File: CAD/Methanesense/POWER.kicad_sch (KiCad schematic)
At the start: 22 parts, among them J1 USB_C_Receptacle_USB2.0_14P, SW3 KMR223GLFG, U1 AP63205WU, U3 nPM1300-QEXX, U4 AP131-20, U7 FT230XQ

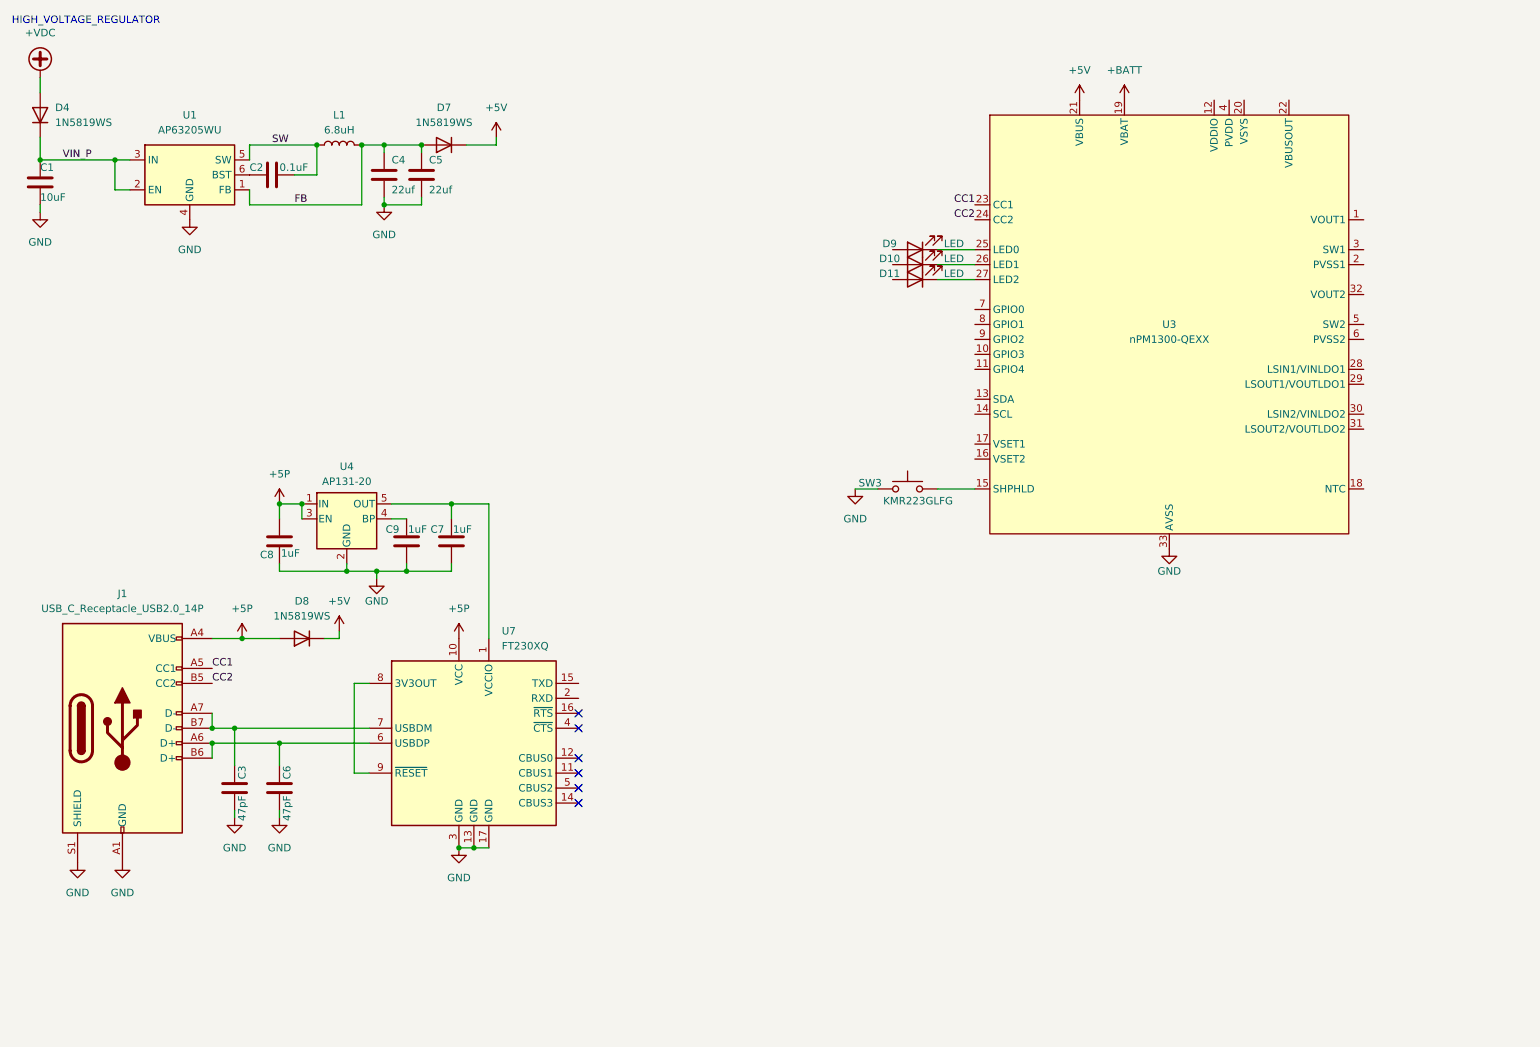
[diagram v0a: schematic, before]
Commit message: WIP
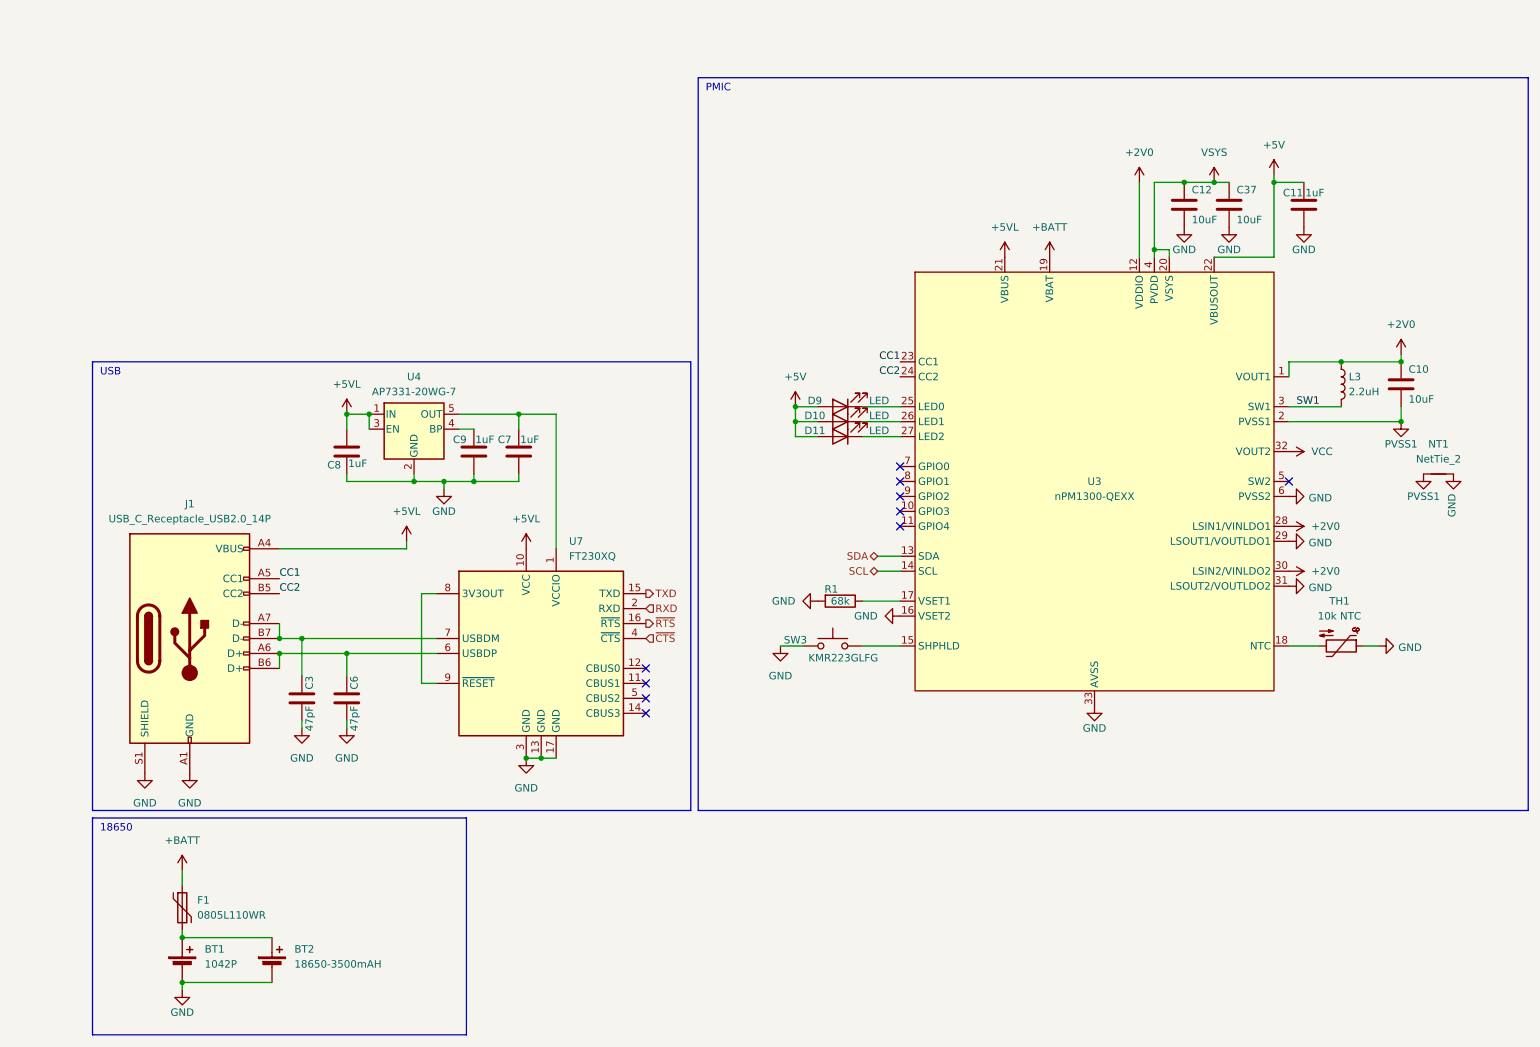
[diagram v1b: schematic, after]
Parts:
- removed C1: 10uF, Capacitor_SMD:C_0805_2012Metric, symbol Library:C
- removed C2: 0.1uF, Capacitor_SMD:C_0402_1005Metric, symbol Library:C
- removed C4, C5: 22uf, Capacitor_SMD:C_0402_1005Metric, symbol Library:C
- removed D4, D7, D8: 1N5819WS, Diode_SMD:D_SOD-323, symbol Library:1N4148WS
- removed L1: 6.8uH, Inductor_SMD:L_1008_2520Metric, symbol Device:L
- removed U1: AP63205WU, Package_TO_SOT_SMD:TSOT-23-6, symbol Regulator_Switching:AP63201WU
- added BT1: 1042P, Battery:BatteryHolder_MPD_BH-18650-PC2, symbol Device:Battery_Cell
- added BT2: 18650-3500mAH, symbol Device:Battery_Cell
- added C10, C12, C37: 10uF, Capacitor_SMD:C_0805_2012Metric, symbol Library:C
- added C11: 1uF, Capacitor_SMD:C_0603_1608Metric, symbol Library:C
- added F1: 0805L110WR, Resistor_SMD:R_1206_3216Metric, symbol Device:Polyfuse
- added L3: 2.2uH, Inductor_SMD:L_1008_2520Metric, symbol Device:L
- added NT1: NetTie_2, esprelay:Viatie, symbol Device:NetTie_2
- added R1: 68k, Resistor_SMD:R_0603_1608Metric, symbol Library:R
- added TH1: 10k NTC, Resistor_SMD:R_0603_1608Metric, symbol Device:Thermistor_NTC
- C3, C6, C7, C8, C9: footprint Capacitor_SMD:C_0402_1005Metric -> Capacitor_SMD:C_0603_1608Metric
- D10, D11, D9: footprint (none) -> LED_SMD:LED_0603_1608Metric
- J1: footprint (none) -> Methanesense:USB_C_Receptacle_HCTL_HC-TYPE-C-16P-01A
- U4: value AP131-20 -> AP7331-20WG-7
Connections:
- net +5V: now also D10.2 (A), D11.2 (A), D9.2 (A), U3.22 (VBUSOUT), C11.1; no longer U3.21 (VBUS)
- net +BATT: now also F1.1
- net GND: now also U3.16 (VSET2), U3.29 (LSOUT1/VOUTLDO1), U3.31 (LSOUT2/VOUTLDO2), U3.6 (PVSS2), BT1.2 (-), BT2.2 (-), C11.2, C12.2, C37.2, NT1.2, R1.2, TH1.1
- net TXD: now reaches U7.15 (TXD)
- net ~{RTS}: now reaches U7.16 (~{RTS})
- net RXD: now reaches U7.2 (RXD)
- net ~{CTS}: now reaches U7.4 (~{CTS})
- net +2V0: now reaches U3.1 (VOUT1)
- net +2V0: now also U3.12 (VDDIO), U3.28 (LSIN1/VINLDO1), U3.30 (LSIN2/VINLDO2), C10.1, L3.1
- net SDA: now reaches U3.13 (SDA)
- net SCL: now reaches U3.14 (SCL)
- net at U3.17 (VSET1): now also R1.1
- net at U3.18 (NTC): now also TH1.2
- net PVSS1: now reaches U3.2 (PVSS1)
- net PVSS1: now also C10.2, NT1.1
- net VSYS: now reaches U3.20 (VSYS)
- net VSYS: now also U3.4 (PVDD), C12.1, C37.1
- net SW1: now reaches U3.3 (SW1)
- net SW1: now also L3.2
- net VCC: now reaches U3.32 (VOUT2)
- net +5P renamed +5VL
- net +5VL: now also U3.21 (VBUS)
- new net: BT1.1 (+), BT2.1 (+), F1.2
- no-connect marks 6 -> 10
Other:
- note added: "18650"
- note added: "PMIC"
- note added: "USB"
- note removed: "HIGH_VOLTAGE_REGULATOR"
- moved on the sheet: C3, C6, C7, C8, C9, D10, D11, D9, J1, SW3, U3, U4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

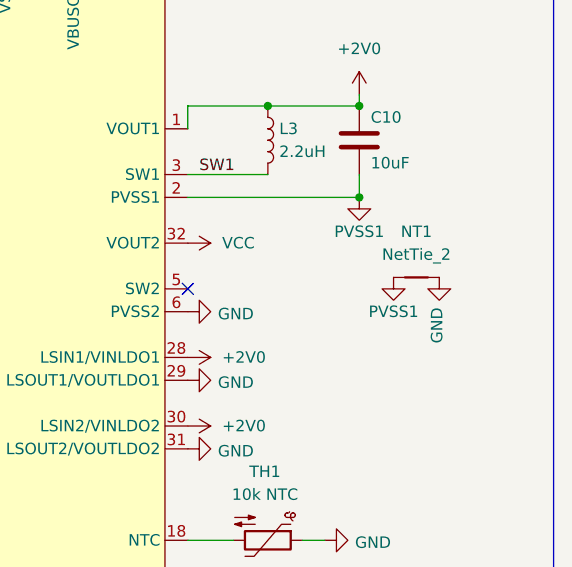
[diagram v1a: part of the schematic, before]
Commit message: WIP
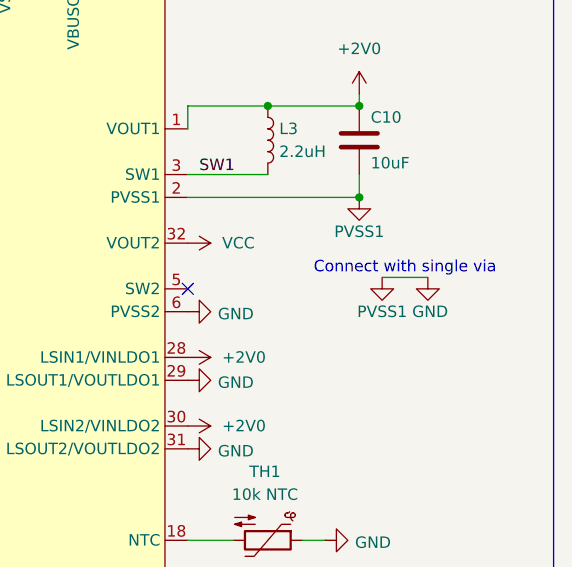
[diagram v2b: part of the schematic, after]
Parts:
- removed NT1: NetTie_2, esprelay:Viatie, symbol Device:NetTie_2
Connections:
- net PVSS1 is gone; now on net GND: C10.2, U3.2 (PVSS1)
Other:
- note added: "Connect with single via"
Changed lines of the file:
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@@
 	(wire
 		(pts
+			(xy 264.16 97.79) (xy 259.08 97.79)
+		)
+		(stroke
+			(width 0)
+			(type default)
+		)
+	)
+	(wire
+		(pts
 			(xy 81.28 90.17) (xy 81.28 87.63)
 		)
@@
 		)
 	)
+	(text "Connect with single via\n"
+		(exclude_from_sim no)
+		(at 261.62 96.774 0)
+		(effects
+			(font
+				(size 1.27 1.27)
+			)
+		)
+	)
 	(text "USB\n"
 		(exclude_from_sim no)
@@
 		)
 		(instances
-			(project ""
+			(project "Methanesense"
 				(path "/51bbc301-ea4a-44e0-84a7-cf42c64443ca/29268011-ceb4-4614-83a3-b1b699d92774"
 					(reference "#PWR028")
@@
 		)
 		(instances
-			(project ""
+			(project "Methanesense"
 				(path "/51bbc301-ea4a-44e0-84a7-cf42c64443ca/29268011-ceb4-4614-83a3-b1b699d92774"
 					(reference "U7")
@@
 		)
 		(instances
-			(project ""
+			(project "Methanesense"
 				(path "/51bbc301-ea4a-44e0-84a7-cf42c64443ca/29268011-ceb4-4614-83a3-b1b699d92774"
 					(reference "TH1")
@@
 		)
 		(instances
-			(project ""
+			(project "Methanesense"
 				(path "/51bbc301-ea4a-44e0-84a7-cf42c64443ca/29268011-ceb4-4614-83a3-b1b699d92774"
 					(reference "U4")
@@
 	)
 	(symbol
-		(lib_id "Device:NetTie_2")
-		(at 262.89 97.79 0)
-		(mirror x)
-		(unit 1)
-		(exclude_from_sim no)
-		(in_bom no)
-		(on_board yes)
-		(dnp no)
-		(property "Reference" "NT1"
-			(at 262.89 92.71 0)
-			(effects
-				(font
-					(size 1.27 1.27)
-				)
-			)
-		)
-		(property "Value" "NetTie_2"
-			(at 262.89 95.25 0)
-			(effects
-				(font
-					(size 1.27 1.27)
-				)
-			)
-		)
-		(property "Footprint" "esprelay:Viatie"
-			(at 262.89 97.79 0)
-			(effects
-				(font
-					(size 1.27 1.27)
-				)
-				(hide yes)
-			)
-		)
-		(property "Datasheet" "~"
-			(at 262.89 97.79 0)
-			(effects
-				(font
-					(size 1.27 1.27)
-				)
-				(hide yes)
-			)
-		)
-		(property "Description" "Net tie, 2 pins"
-			(at 262.89 97.79 0)
-			(effects
-				(font
-					(size 1.27 1.27)
-				)
-				(hide yes)
-			)
-		)
-		(property "TEST" ""
-			(at 262.89 97.79 0)
-			(effects
-				(font
-					(size 1.27 1.27)
-				)
-			)
-		)
-		(pin "2"
-		)
-		(pin "1"
-		)
-		(instances
-			(project ""
-				(path "/51bbc301-ea4a-44e0-84a7-cf42c64443ca/29268011-ceb4-4614-83a3-b1b699d92774"
-					(reference "NT1")
-					(unit 1)
-				)
-			)
-		)
-	)
-	(symbol
 		(lib_id "power:+5VL")
 		(at 107.95 110.49 0)
@@
 	(symbol
 		(lib_id "power:GND")
-		(at 265.43 97.79 0)
+		(at 264.16 97.79 0)
 		(unit 1)
 		(exclude_from_sim no)
@@
 		(dnp no)
 		(property "Reference" "#PWR046"
-			(at 265.43 104.14 0)
+			(at 264.16 104.14 0)
 			(effects
 				(font
@@
 		)
 		(property "Value" "GND"
-			(at 265.176 103.124 90)
+			(at 264.414 101.6 0)
 			(effects
 				(font
@@
 		)
 		(property "Footprint" ""
-			(at 265.43 97.79 0)
+			(at 264.16 97.79 0)
 			(effects
 				(font
@@
 		)
 		(property "Datasheet" ""
-			(at 265.43 97.79 0)
+			(at 264.16 97.79 0)
 			(effects
 				(font
@@
 		)
 		(property "Description" ""
-			(at 265.43 97.79 0)
+			(at 264.16 97.79 0)
 			(effects
 				(font
@@
 		)
 		(instances
-			(project ""
+			(project "Methanesense"
 				(path "/51bbc301-ea4a-44e0-84a7-cf42c64443ca/29268011-ceb4-4614-83a3-b1b699d92774"
 					(reference "#PWR027")
@@
 		)
 		(instances
-			(project ""
+			(project "Methanesense"
 				(path "/51bbc301-ea4a-44e0-84a7-cf42c64443ca/29268011-ceb4-4614-83a3-b1b699d92774"
 					(reference "J1")
@@
 	(symbol
 		(lib_id "power:GND")
-		(at 260.35 97.79 0)
+		(at 259.08 97.79 0)
 		(unit 1)
 		(exclude_from_sim no)
@@
 		(dnp no)
 		(property "Reference" "#PWR045"
-			(at 260.35 104.14 0)
+			(at 259.08 104.14 0)
 			(effects
 				(font
@@
 		)
 		(property "Value" "PVSS1"
-			(at 260.35 101.6 0)
+			(at 259.08 101.6 0)
 			(effects
 				(font
@@
 		)
 		(property "Footprint" ""
-			(at 260.35 97.79 0)
+			(at 259.08 97.79 0)
 			(effects
 				(font
@@
 		)
 		(property "Datasheet" ""
-			(at 260.35 97.79 0)
+			(at 259.08 97.79 0)
 			(effects
 				(font
@@
 		)
 		(property "Description" ""
-			(at 260.35 97.79 0)
+			(at 259.08 97.79 0)
 			(effects
 				(font
@@
 		)
 		(property "TEST" ""
-			(at 260.35 97.79 0)
+			(at 259.08 97.79 0)
 			(effects
 				(font
@@
 		)
 		(instances
-			(project ""
+			(project "Methanesense"
 				(path "/51bbc301-ea4a-44e0-84a7-cf42c64443ca/29268011-ceb4-4614-83a3-b1b699d92774"
 					(reference "U3")
@@
 		)
 		(instances
-			(project ""
+			(project "Methanesense"
 				(path "/51bbc301-ea4a-44e0-84a7-cf42c64443ca/29268011-ceb4-4614-83a3-b1b699d92774"
 					(reference "#PWR053")
